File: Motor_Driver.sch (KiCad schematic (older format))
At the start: 42 parts, among them J1 Conn_01x04_Male, J2 Conn_01x40_Male, J3 Conn_01x02_Female, Q1 Q_NMOS_SGD, Q2 Q_NMOS_SGD, Q3 Q_NMOS_SGD, Q4 Q_NMOS_SGD, U1 NJM7812, U2 Si8274(DFN-14), U3 Si8274(DFN-14)

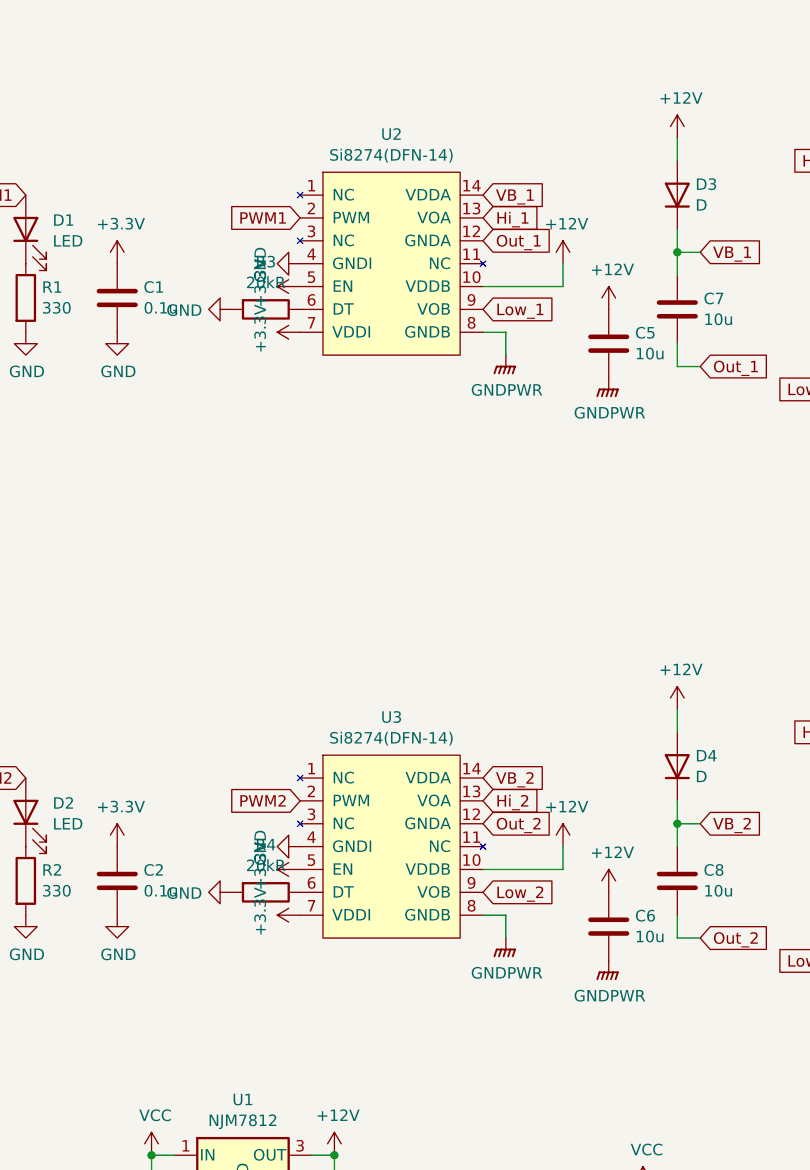
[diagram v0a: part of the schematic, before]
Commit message: 0.1 first
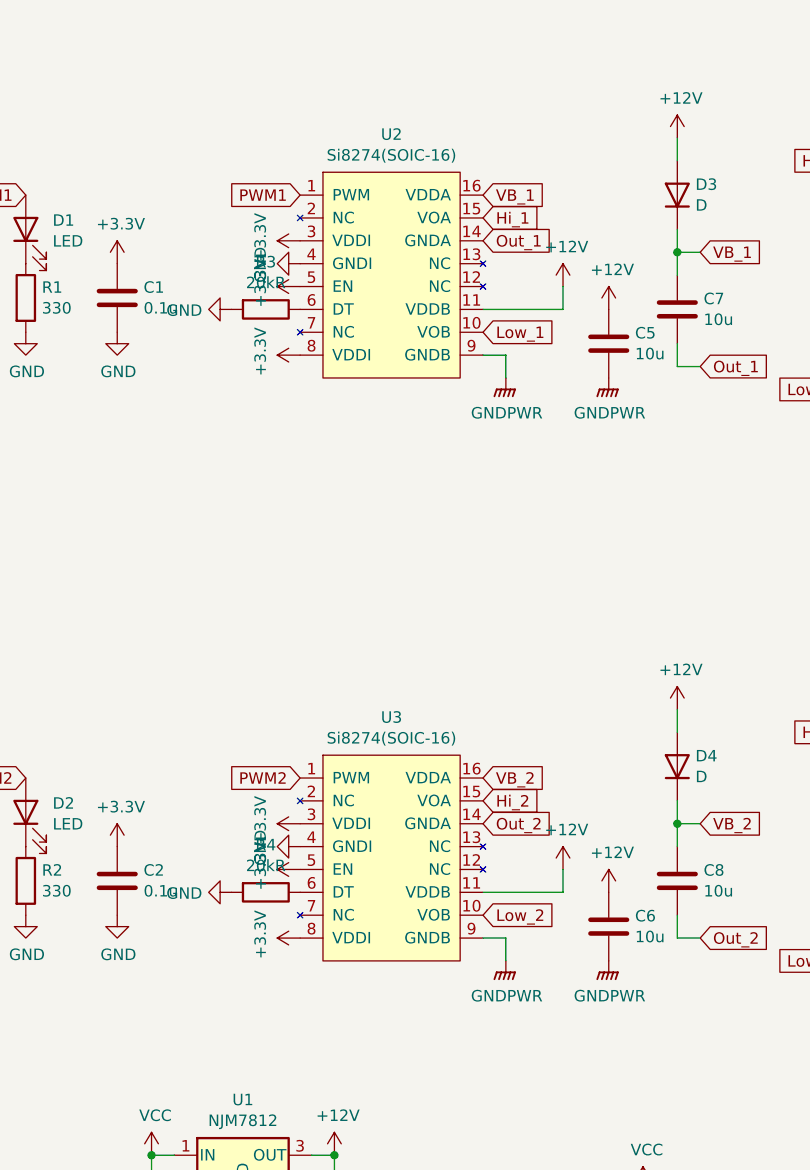
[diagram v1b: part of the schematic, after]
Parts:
- removed U2, U3: Si8274(DFN-14), Package_DFN_QFN_additional:DFN-14_4.9x4.9mm_P0.65mm, symbol Si8274:Si8274(DFN-14)
- added U2, U3: Si8274(SOIC-16), Package_SO:SOIC-16_3.9x9.9mm_P1.27mm, symbol Si8274:Si8274(SOIC-16)
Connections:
- net +12V: now also U2.11 (VDDB), U3.11 (VDDB)
- net +3V3: now also U2.3 (VDDI), U2.5 (EN), U2.8 (VDDI), U3.3 (VDDI), U3.5 (EN), U3.8 (VDDI)
- net GND: now also U2.4 (GNDI), U3.4 (GNDI)
- net GNDPWR: now also U2.9 (GNDB), U3.9 (GNDB)
- net Hi_1: now also U2.15 (VOA)
- net Hi_2: now also U3.15 (VOA)
- net Low_1: now also U2.10 (VOB)
- net Low_2: now also U3.10 (VOB)
- net Out_1: now also U2.14 (GNDA)
- net Out_2: now also U3.14 (GNDA)
- net PWM1: now also U2.1 (PWM)
- net PWM2: now also U3.1 (PWM)
- net VB_1: now also U2.16 (VDDA)
- net VB_2: now also U3.16 (VDDA)
- net at R4.1: now also U3.6 (DT)
- net at R3.1: now also U2.6 (DT)
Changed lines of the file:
@@
 EESchema Schematic File Version 4
+LIBS:Motor_Driver-cache
 EELAYER 30 0
 EELAYER END
@@
 Text GLabel 9000 1500 0    50   Input ~ 0
 Hi_1
-Text GLabel 7400 2150 2    50   Input ~ 0
+Text GLabel 7400 2250 2    50   Input ~ 0
 Low_1
 Text GLabel 9000 2500 0    50   Input ~ 0
@@
 Text GLabel 9000 4000 0    50   Input ~ 0
 Hi_2
-Text GLabel 7400 4700 2    50   Input ~ 0
+Text GLabel 7400 4800 2    50   Input ~ 0
 Low_2
 Text GLabel 9000 5000 0    50   Input ~ 0
@@
 	10100 5250 10100 5400
 $Comp
+L Si8274:Si8274(SOIC-16) U2
+U 1 1 600B4EB8
+P 7000 2000
+F 0 "U2" H 7000 2615 50  0000 C CNN
+F 1 "Si8274(SOIC-16)" H 7000 2524 50  0000 C CNN
+F 2 "Package_SO:SOIC-16_3.9x9.9mm_P1.27mm" H 7000 1450 50  0001 C CNN
+F 3 "" H 7000 1450 50  0001 C CNN
+	1    7000 2000
+	1    0    0    -1
+$EndComp
+$Comp
+L Si8274:Si8274(SOIC-16) U3
+U 1 1 600B697E
+P 7000 4550
+F 0 "U3" H 7000 5165 50  0000 C CNN
+F 1 "Si8274(SOIC-16)" H 7000 5074 50  0000 C CNN
+F 2 "Package_SO:SOIC-16_3.9x9.9mm_P1.27mm" H 7000 4000 50  0001 C CNN
+F 3 "" H 7000 4000 50  0001 C CNN
+	1    7000 4550
+	1    0    0    -1
+$EndComp
+$Comp
 L Device:Q_NMOS_SGD Q1
 U 1 1 600D89C7
@@
 $EndComp
 Wire Wire Line
-	7400 4800 7500 4800
-Wire Wire Line
-	7500 4800 7500 4900
-Wire Wire Line
-	7400 2250 7500 2250
-Wire Wire Line
-	7500 2250 7500 2350
-Wire Wire Line
-	7750 2050 7750 1950
-Wire Wire Line
-	7750 4600 7750 4500
+	7400 4900 7500 4900
+Wire Wire Line
+	7500 4900 7500 5000
+Wire Wire Line
+	7400 2350 7500 2350
+Wire Wire Line
+	7500 2350 7500 2450
+Wire Wire Line
+	7750 2150 7750 2050
+Wire Wire Line
+	7750 4700 7750 4600
 $Comp
 L power:GNDPWR #PWR023
 U 1 1 600F8A75
-P 7500 4900
-F 0 "#PWR023" H 7500 4700 50  0001 C CNN
-F 1 "GNDPWR" H 7504 4746 50  0000 C CNN
-F 2 "" H 7500 4850 50  0001 C CNN
-F 3 "" H 7500 4850 50  0001 C CNN
-	1    7500 4900
+P 7500 5000
+F 0 "#PWR023" H 7500 4800 50  0001 C CNN
+F 1 "GNDPWR" H 7504 4846 50  0000 C CNN
+F 2 "" H 7500 4950 50  0001 C CNN
+F 3 "" H 7500 4950 50  0001 C CNN
+	1    7500 5000
 	1    0    0    -1
 $EndComp
@@
 L power:GNDPWR #PWR022
 U 1 1 60101F3B
-P 7500 2350
-F 0 "#PWR022" H 7500 2150 50  0001 C CNN
-F 1 "GNDPWR" H 7504 2196 50  0000 C CNN
-F 2 "" H 7500 2300 50  0001 C CNN
-F 3 "" H 7500 2300 50  0001 C CNN
-	1    7500 2350
+P 7500 2450
+F 0 "#PWR022" H 7500 2250 50  0001 C CNN
+F 1 "GNDPWR" H 7504 2296 50  0000 C CNN
+F 2 "" H 7500 2400 50  0001 C CNN
+F 3 "" H 7500 2400 50  0001 C CNN
+	1    7500 2450
 	1    0    0    -1
 $EndComp
@@
 L power:+12V #PWR024
 U 1 1 601069A2
-P 7750 1950
-F 0 "#PWR024" H 7750 1800 50  0001 C CNN
-F 1 "+12V" H 7765 2123 50  0000 C CNN
-F 2 "" H 7750 1950 50  0001 C CNN
-F 3 "" H 7750 1950 50  0001 C CNN
-	1    7750 1950
+P 7750 2050
+F 0 "#PWR024" H 7750 1900 50  0001 C CNN
+F 1 "+12V" H 7765 2223 50  0000 C CNN
+F 2 "" H 7750 2050 50  0001 C CNN
+F 3 "" H 7750 2050 50  0001 C CNN
+	1    7750 2050
 	1    0    0    -1
 $EndComp
@@
 L power:+12V #PWR025
 U 1 1 6010AEFC
-P 7750 4500
-F 0 "#PWR025" H 7750 4350 50  0001 C CNN
-F 1 "+12V" H 7765 4673 50  0000 C CNN
-F 2 "" H 7750 4500 50  0001 C CNN
-F 3 "" H 7750 4500 50  0001 C CNN
-	1    7750 4500
-	1    0    0    -1
-$EndComp
-Wire Wire Line
-	7400 4600 7750 4600
-Wire Wire Line
-	7400 2050 7750 2050
+P 7750 4600
+F 0 "#PWR025" H 7750 4450 50  0001 C CNN
+F 1 "+12V" H 7765 4773 50  0000 C CNN
+F 2 "" H 7750 4600 50  0001 C CNN
+F 3 "" H 7750 4600 50  0001 C CNN
+	1    7750 4600
+	1    0    0    -1
+$EndComp
+Wire Wire Line
+	7400 4700 7750 4700
+Wire Wire Line
+	7400 2150 7750 2150
 $Comp
 L power:+3.3V #PWR016
 U 1 1 6012309A
-P 6600 2250
-F 0 "#PWR016" H 6600 2100 50  0001 C CNN
-F 1 "+3.3V" H 6615 2423 50  0000 C CNN
-F 2 "" H 6600 2250 50  0001 C CNN
-F 3 "" H 6600 2250 50  0001 C CNN
-	1    6600 2250
+P 6600 2350
+F 0 "#PWR016" H 6600 2200 50  0001 C CNN
+F 1 "+3.3V" H 6615 2523 50  0000 C CNN
+F 2 "" H 6600 2350 50  0001 C CNN
+F 3 "" H 6600 2350 50  0001 C CNN
+	1    6600 2350
+	0    -1   -1   0
+$EndComp
+$Comp
+L power:+3.3V #PWR013
+U 1 1 601277F7
+P 6600 1850
+F 0 "#PWR013" H 6600 1700 50  0001 C CNN
+F 1 "+3.3V" H 6615 2023 50  0000 C CNN
+F 2 "" H 6600 1850 50  0001 C CNN
+F 3 "" H 6600 1850 50  0001 C CNN
+	1    6600 1850
 	0    -1   -1   0
 $EndComp
@@
 L power:+3.3V #PWR020
 U 1 1 6012BF35
-P 6600 4800
-F 0 "#PWR020" H 6600 4650 50  0001 C CNN
-F 1 "+3.3V" H 6615 4973 50  0000 C CNN
-F 2 "" H 6600 4800 50  0001 C CNN
-F 3 "" H 6600 4800 50  0001 C CNN
-	1    6600 4800
+P 6600 4900
+F 0 "#PWR020" H 6600 4750 50  0001 C CNN
+F 1 "+3.3V" H 6615 5073 50  0000 C CNN
+F 2 "" H 6600 4900 50  0001 C CNN
+F 3 "" H 6600 4900 50  0001 C CNN
+	1    6600 4900
+	0    -1   -1   0
+$EndComp
+$Comp
+L power:+3.3V #PWR017
+U 1 1 6013068D
+P 6600 4400
+F 0 "#PWR017" H 6600 4250 50  0001 C CNN
+F 1 "+3.3V" H 6615 4573 50  0000 C CNN
+F 2 "" H 6600 4400 50  0001 C CNN
+F 3 "" H 6600 4400 50  0001 C CNN
+	1    6600 4400
 	0    -1   -1   0
 $EndComp
@@
 	0    1    1    0
 $EndComp
-Text GLabel 6600 1750 0    50   Input ~ 0
+Text GLabel 6600 1650 0    50   Input ~ 0
 PWM1
-Text GLabel 6600 4300 0    50   Input ~ 0
+Text GLabel 6600 4200 0    50   Input ~ 0
 PWM2
 $Comp
@@
 Wire Wire Line
 	10100 4300 10100 4500
-$Comp
-L Si8274:Si8274(DFN-14) U2
-U 1 1 6141E1DE
-P 7000 1950
-F 0 "U2" H 7000 2515 50  0000 C CNN
-F 1 "Si8274(DFN-14)" H 7000 2424 50  0000 C CNN
-F 2 "Package_DFN_QFN_additional:DFN-14_4.9x4.9mm_P0.65mm" H 7000 1450 50  0001 C CNN
-F 3 "" H 7000 1450 50  0001 C CNN
-	1    7000 1950
-	1    0    0    -1
-$EndComp
-$Comp
-L Si8274:Si8274(DFN-14) U3
-U 1 1 61439B83
-P 7000 4500
-F 0 "U3" H 7000 5065 50  0000 C CNN
-F 1 "Si8274(DFN-14)" H 7000 4974 50  0000 C CNN
-F 2 "Package_DFN_QFN_additional:DFN-14_4.9x4.9mm_P0.65mm" H 7000 4000 50  0001 C CNN
-F 3 "" H 7000 4000 50  0001 C CNN
-	1    7000 4500
-	1    0    0    -1
-$EndComp
 $EndSCHEMATC
